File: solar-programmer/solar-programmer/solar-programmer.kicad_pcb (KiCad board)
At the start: 2 copper layers, 30 x 65 mm, 22 parts, among them J1 Raspberry_Pi_2_3, J2 6P6C, J3 TC2030, SW1 SW_Push

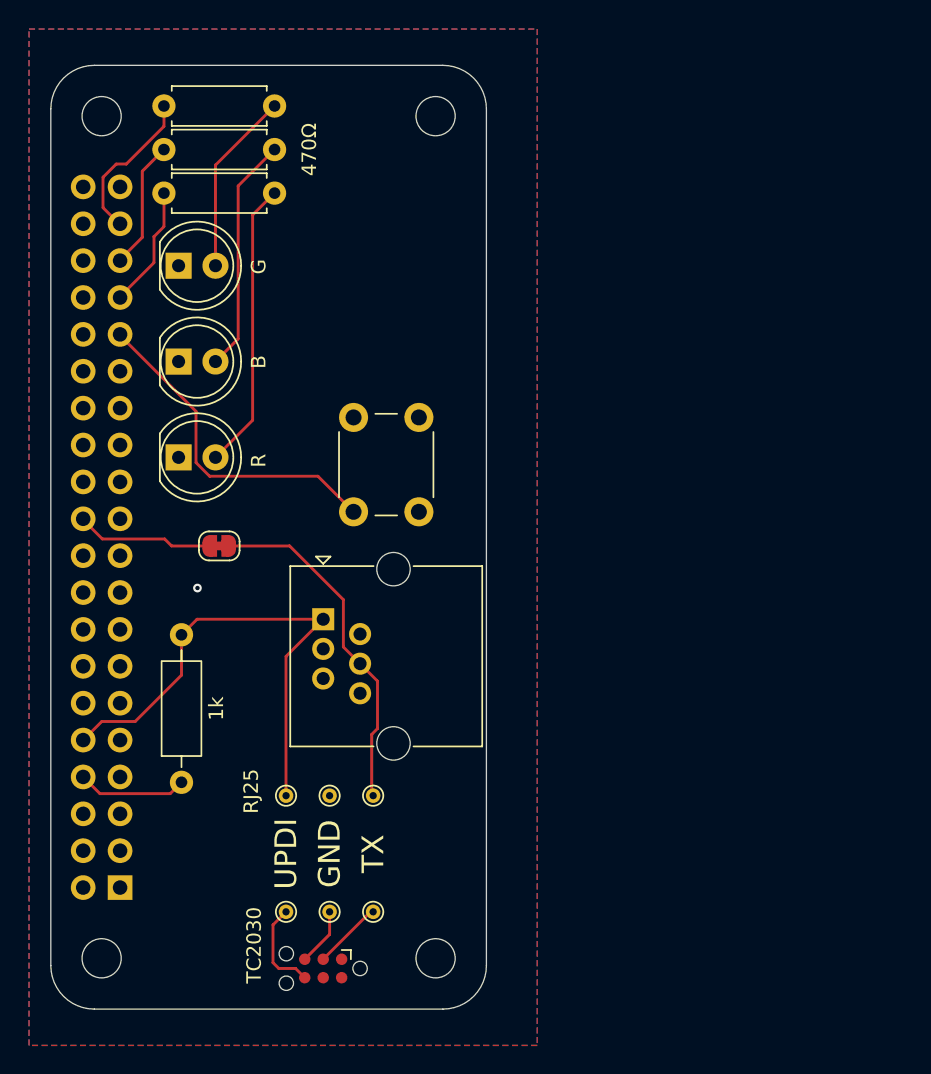
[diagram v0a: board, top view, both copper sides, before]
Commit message: Getting ready for v0.3.0
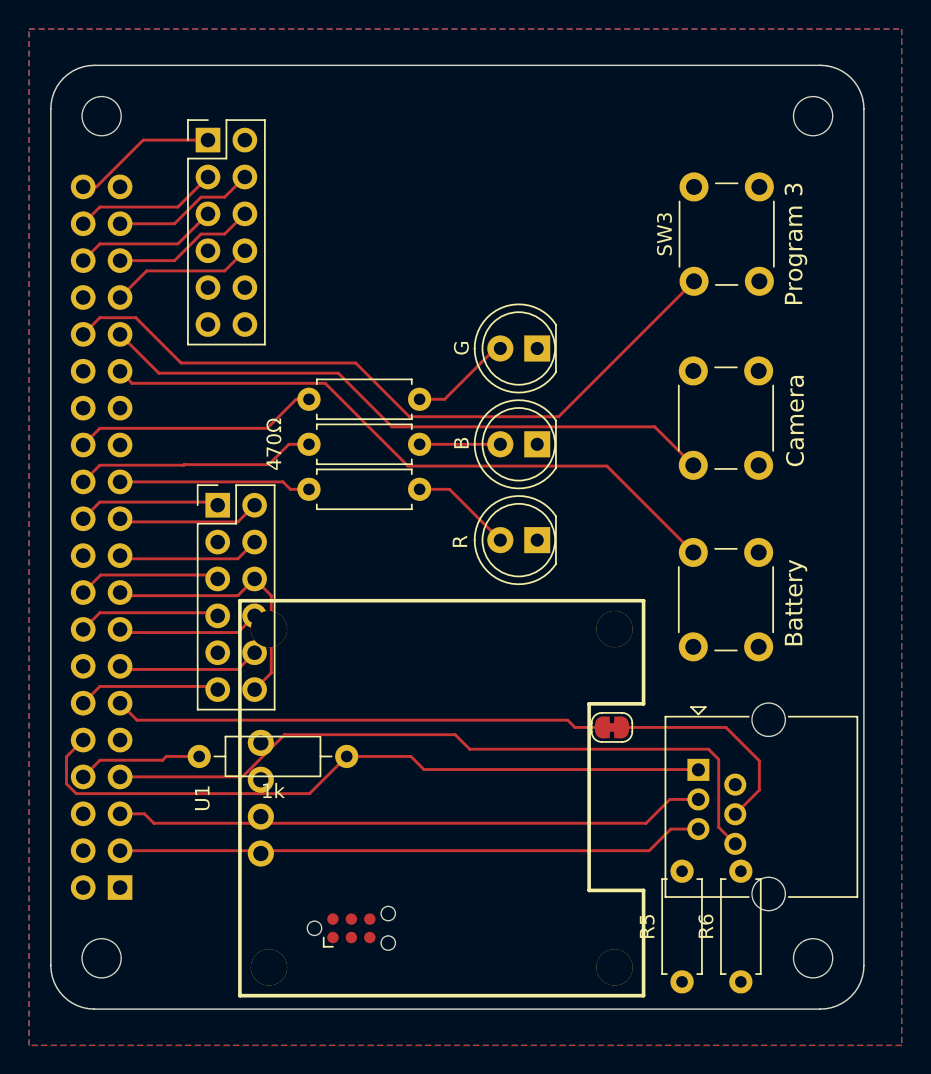
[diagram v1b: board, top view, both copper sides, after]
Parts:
- removed TP1, TP2, TP3, TP4, TP5, TP6: TestPoint, TestPoint:TestPoint_THTPad_D1.0mm_Drill0.5mm
- added J5: Conn_02x06_Odd_Even, Connector_PinHeader_2.54mm:PinHeader_2x06_P2.54mm_Vertical, F.Cu at (8.00, -2.21)
- added J6: Conn_02x06_Odd_Even, Connector_PinHeader_2.54mm:PinHeader_2x06_P2.54mm_Vertical, F.Cu at (7.33, -27.4)
- added R5: 10k, Resistor_THT:R_Axial_DIN0207_L6.3mm_D2.5mm_P7.62mm_Horizontal, F.Cu at (40.0, 30.6)
- added R6: 10k, Resistor_THT:R_Axial_DIN0207_L6.3mm_D2.5mm_P7.62mm_Horizontal, F.Cu at (44.0, 30.6)
- added SW2: SW_Push, cacophony-library:SW_PUSH_6mm_11mmh, F.Cu at (43.0, -8.20)
- added SW3: SW_Push, cacophony-library:SW_PUSH_6mm_11mmh, F.Cu at (43.0, -20.9)
- added U1: HS96L03W2C03, cacophony-library:OLED-TH_L27.8-W27.2-P2.54_C9900033791, F.Cu at (11.0, 18.0)
- J1: footprint cacophony-library:rpi-zero-throughhole-socket -> cacophony-library:rpi-3-hat; moved to F.Cu
- moved JP1 29.8 mm to (35.1, 13.1)
- moved J2 27.8 mm to (41.1, 16.0)
- moved H2 26.0 mm to (49.0, -29.0)
- moved H4 26.0 mm to (49.0, 29.0)
- moved D1 25.3 mm to (30.0, 0.20), turned to 180 degrees
- moved D2 25.3 mm to (30.0, -13.0), turned to 180 degrees
- moved D3 25.3 mm to (30.0, -6.40), turned to 180 degrees
- moved SW1 25.2 mm to (43.0, 4.30)
- moved R2 22.7 mm to (14.3, -3.30)
- moved R4 22.6 mm to (14.3, -6.40)
- moved R3 22.5 mm to (14.3, -9.50)
- moved J3 3.38 mm to (17.2, 26.9), turned to 0 degrees
- moved R1 2.16 mm to (6.72, 15.1), turned to 0 degrees
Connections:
- J1 pad 1: unconnected-(J1-3V3-Pad1)_1 -> +3.3V
- J1 pad 11: unconnected-(J1-GPIO17-Pad11) -> Net-(J1-GPIO17)
- J1 pad 12: unconnected-(J1-GPIO18/PWM0-Pad12) -> GPIO18
- J1 pad 13: unconnected-(J1-GPIO27-Pad13) -> GPIO27
- J1 pad 15: unconnected-(J1-GPIO22-Pad15) -> GPIO22
- J1 pad 16: unconnected-(J1-GPIO23-Pad16) -> GPIO23
- J1 pad 17: unconnected-(J1-3V3-Pad1) -> +3.3V
- J1 pad 18: unconnected-(J1-GPIO24-Pad18) -> GPIO24
- J1 pad 19: unconnected-(J1-MOSI0/GPIO10-Pad19) -> GPIO10
- J1 pad 2: unconnected-(J1-5V-Pad2) -> +5V
- J1 pad 21: unconnected-(J1-MISO0/GPIO9-Pad21) -> GPIO9
- J1 pad 22: /RPI_RX -> GPIO25
- J1 pad 23: unconnected-(J1-SCLK0/GPIO11-Pad23) -> LED_R
- J1 pad 24: unconnected-(J1-~{CE0}/GPIO8-Pad24) -> LED_B
- J1 pad 26: unconnected-(J1-~{CE1}/GPIO7-Pad26) -> LED_G
- J1 pad 29: unconnected-(J1-GCLK1/GPIO5-Pad29) -> PROGRAM_CAMERA
- J1 pad 3: unconnected-(J1-SDA/GPIO2-Pad3) -> SDA
- J1 pad 31: BUTTON -> PROGRAM_BATTERY_BUTTON
- J1 pad 32: unconnected-(J1-PWM0/GPIO12-Pad32) -> PROGRAM_TRAP
- J1 pad 33: LED_R -> GPIO13
- J1 pad 35: LED_B -> GPIO19
- J1 pad 36: unconnected-(J1-GPIO16-Pad36) -> GPIO16
- J1 pad 37: LED_G -> GPIO26
- J1 pad 38: unconnected-(J1-GPIO20/MOSI1-Pad38) -> GPIO20
- J1 pad 4: unconnected-(J1-5V-Pad2)_1 -> +5V
- J1 pad 40: unconnected-(J1-GPIO21/SCLK1-Pad40) -> GPIO21
- J1 pad 5: unconnected-(J1-SCL/GPIO3-Pad5) -> SCL
- J1 pad 7: unconnected-(J1-GCLK0/GPIO4-Pad7) -> EEPROM_~{WC}
- J2 pad 3: unconnected-(J2-Pad3) -> SCL
- J2 pad 5: unconnected-(J2-Pad5) -> SDA
- J2 pad 6: unconnected-(J2-Pad6) -> EEPROM_~{WC}
- J3 pad 1: unconnected-(J3-Pad1) -> EEPROM_~{WC}_TEST
- J3 pad 2: unconnected-(J3-Pad2) -> SDA_TEST
- J3 pad 4: unconnected-(J3-Pad4) -> SCL_TEST
- JP1 pad 2: /RPI_RX -> Net-(J1-GPIO17)
- SW1 pad 1: BUTTON -> PROGRAM_CAMERA
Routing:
- net EEPROM_~{WC}: track 0.00 -> 49.4 mm
- net PROGRAM_TRAP: track 0.00 -> 49.2 mm
- net PROGRAM_CAMERA: track 0.00 -> 44.6 mm
- net PROGRAM_BATTERY_BUTTON: track 0.00 -> 43.2 mm
- net SCL: track 0.00 -> 40.8 mm
- net SDA: track 0.00 -> 40.4 mm
- net Net-(J1-GPIO17): track 0.00 -> 33.9 mm
- net BUTTON: track 23.3 -> 0.00 mm
- net +3.3V: track 0.00 -> 18.4 mm
- net UPDI: track 34.8 -> 48.7 mm
- net Net-(D1-A): track 19.9 -> 7.01 mm
- net Net-(D3-A): track 16.3 -> 5.50 mm
- net GPIO21: track 0.00 -> 9.93 mm
- net GPIO26: track 0.00 -> 9.93 mm
- net GPIO20: track 0.00 -> 9.93 mm
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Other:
- board size 30 x 65 mm -> 56 x 65 mm
- board text added: "Battery"
- board text added: "Camera"
- board text added: "Program 3"
- board text removed: "GND"
- board text removed: "RJ25"
- board text removed: "TC2030"
- board text removed: "TX"
- board text removed: "UPDI"
